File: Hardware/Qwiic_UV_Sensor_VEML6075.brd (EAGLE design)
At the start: 25.4 x 25.4 mm, 35 parts, among them J3 PTH, U1 VEML6075

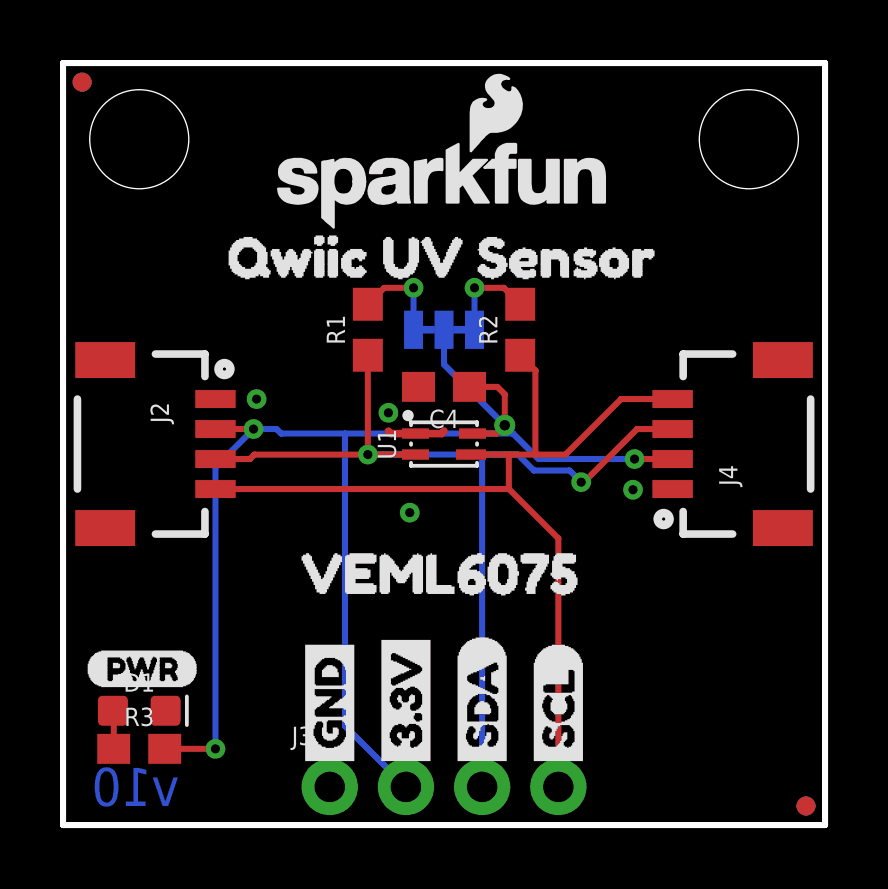
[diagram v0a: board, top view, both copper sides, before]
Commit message: post checklist changes
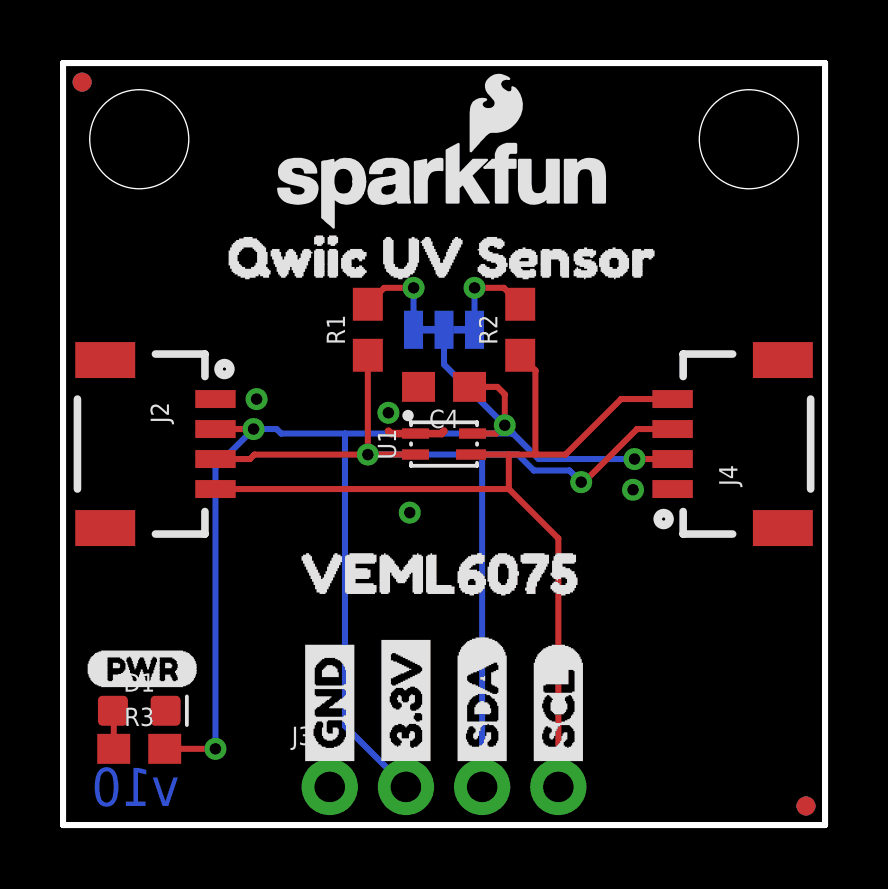
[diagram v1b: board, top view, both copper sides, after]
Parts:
- U1: device Qwiic_UV_Sensor_VEML6075:VEML6075_A3OP -> SparkFun-Sensors:VEML6075_A3OP
